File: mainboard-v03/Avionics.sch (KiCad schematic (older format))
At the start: 42 parts, among them J10 Conn_01x03, J8 Conn_01x09, J9 Conn_01x05, SW1 KMR231NG LFS, U1 MAX706RS-T, U2 ATSAMD51J20A-AU, U3 LSM9DS1, Y1 32.768kHz

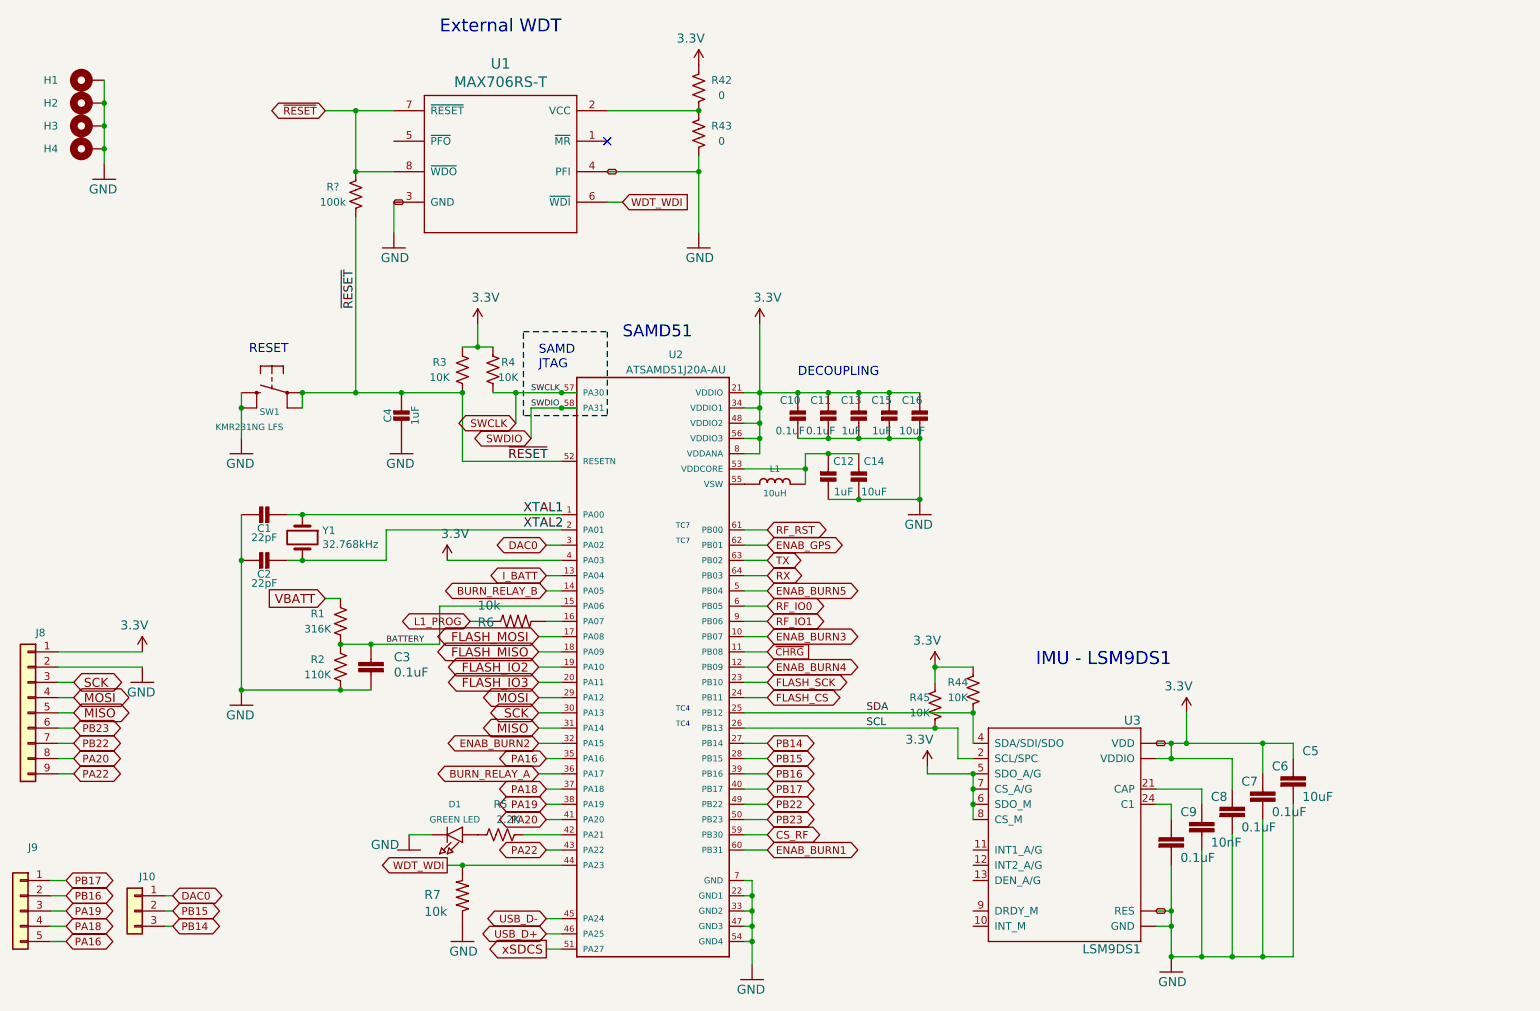
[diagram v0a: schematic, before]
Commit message: schematic organizing
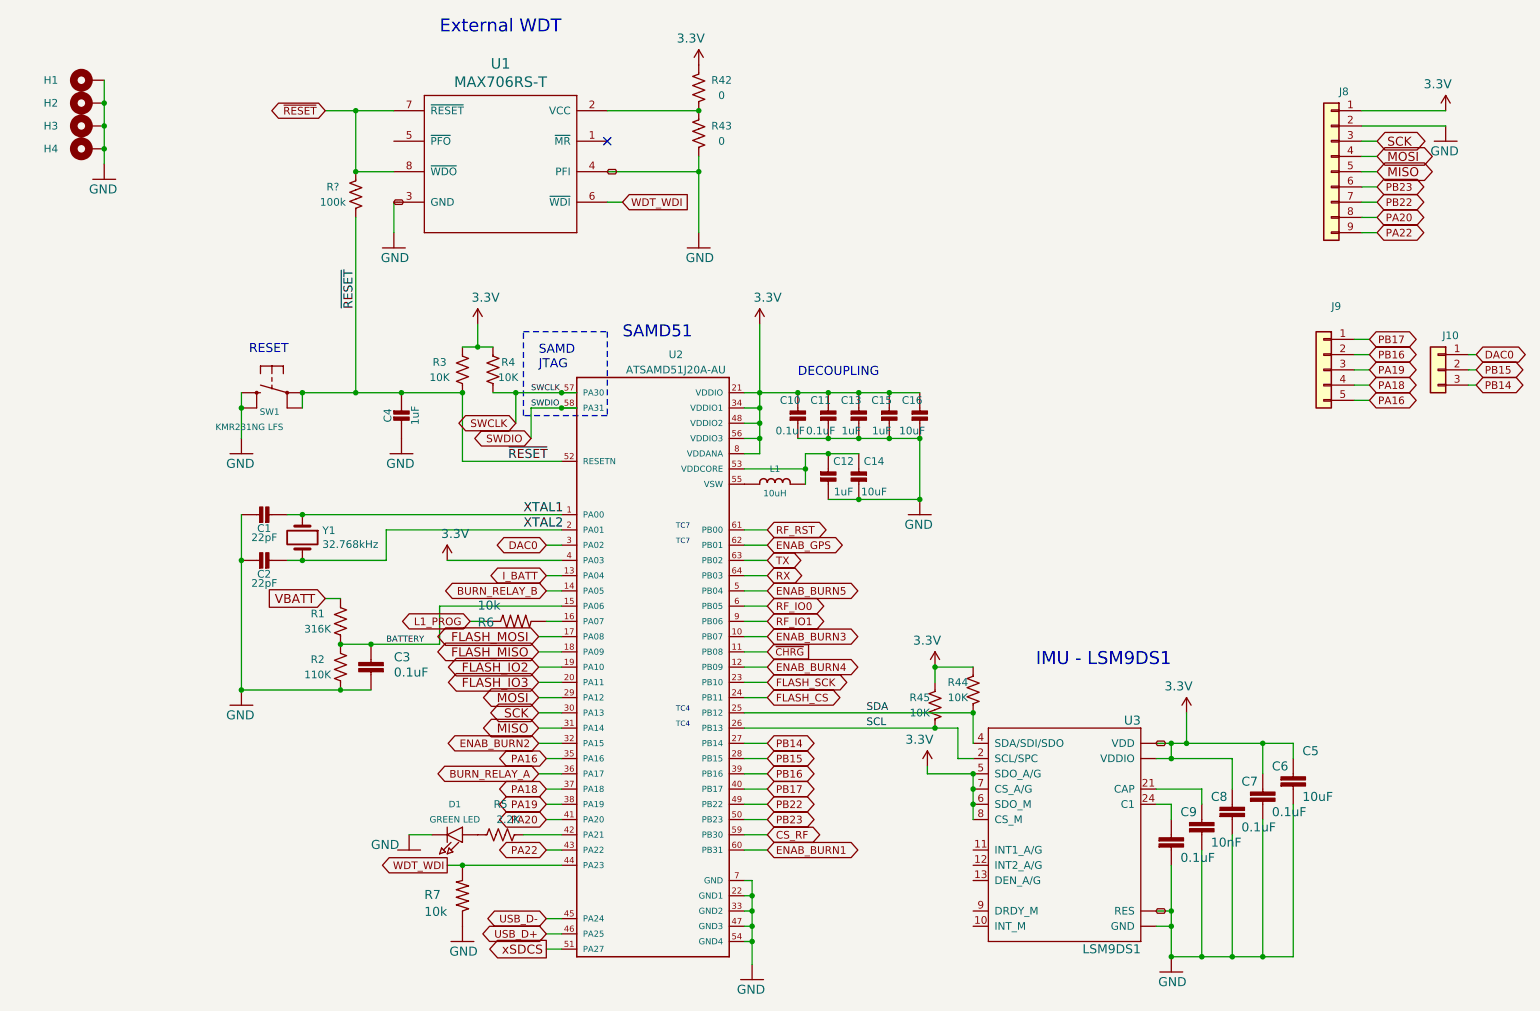
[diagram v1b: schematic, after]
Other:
- moved on the sheet: J10, J8, J9
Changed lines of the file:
@@
 Text GLabel 4600 5850 0    50   BiDi ~ 0
 PA19
-Text GLabel 1500 5150 2    59   BiDi ~ 0
+Text GLabel 10050 1600 2    59   BiDi ~ 0
 MOSI
-Text GLabel 1500 5050 2    59   BiDi ~ 0
+Text GLabel 10050 1500 2    59   BiDi ~ 0
 SCK
-Text GLabel 1500 5250 2    59   BiDi ~ 0
+Text GLabel 10050 1700 2    59   BiDi ~ 0
 MISO
 Wire Wire Line
-	1500 5150 1400 5150
-Wire Wire Line
-	1500 5050 1400 5050
-Wire Wire Line
-	1500 5250 1400 5250
+	10050 1600 9950 1600
+Wire Wire Line
+	10050 1500 9950 1500
+Wire Wire Line
+	10050 1700 9950 1700
 Wire Wire Line
 	6050 4850 5900 4850
@@
 	3350 1300 3150 1300
 Wire Wire Line
-	1400 5550 1500 5550
-Text GLabel 1500 5550 2    50   BiDi ~ 0
+	9950 2000 10050 2000
+Text GLabel 10050 2000 2    50   BiDi ~ 0
 PA20
 Wire Wire Line
-	1400 5650 1500 5650
-Text GLabel 1500 5650 2    50   BiDi ~ 0
+	9950 2100 10050 2100
+Text GLabel 10050 2100 2    50   BiDi ~ 0
 PA22
 Wire Wire Line
-	1400 5350 1500 5350
-Text GLabel 1500 5350 2    50   BiDi ~ 0
+	9950 1800 10050 1800
+Text GLabel 10050 1800 2    50   BiDi ~ 0
 PB23
 Wire Wire Line
-	1400 5450 1500 5450
-Text GLabel 1500 5450 2    50   BiDi ~ 0
+	9950 1900 10050 1900
+Text GLabel 10050 1900 2    50   BiDi ~ 0
 PB22
 $Comp
 L Connector_Generic:Conn_01x09 J8
 U 1 1 5D3643AA
-P 1200 5250
-F 0 "J8" H 1118 5775 50  0000 C CNN
-F 1 "Conn_01x09" H 1118 5776 50  0001 C CNN
-F 2 "Connector_PinHeader_2.54mm:PinHeader_1x09_P2.54mm_Vertical" H 1200 5250 50  0001 C CNN
-F 3 "~" H 1200 5250 50  0001 C CNN
-	1    1200 5250
+P 9750 1700
+F 0 "J8" H 9668 2225 50  0000 C CNN
+F 1 "Conn_01x09" H 9668 2226 50  0001 C CNN
+F 2 "Connector_PinHeader_2.54mm:PinHeader_1x09_P2.54mm_Vertical" H 9750 1700 50  0001 C CNN
+F 3 "~" H 9750 1700 50  0001 C CNN
+	1    9750 1700
 	-1   0    0    -1
 $EndComp
@@
 L mainboard:3.3V #SUPPLY?
 U 1 0 5D370A56
-P 1950 4850
+P 10500 1300
 AR Path="/5D370A56" Ref="#SUPPLY?"  Part="1"
 AR Path="/5CEC5A72/5D370A56" Ref="#SUPPLY0111"  Part="1"
-F 0 "#SUPPLY0111" H 1950 4850 50  0001 C CNN
-F 1 "3.3V" H 1910 4990 59  0000 L BNN
-F 2 "" H 1950 4850 50  0001 C CNN
-F 3 "" H 1950 4850 50  0001 C CNN
-	1    1950 4850
+F 0 "#SUPPLY0111" H 10500 1300 50  0001 C CNN
+F 1 "3.3V" H 10460 1440 59  0000 L BNN
+F 2 "" H 10500 1300 50  0001 C CNN
+F 3 "" H 10500 1300 50  0001 C CNN
+	1    10500 1300
 	-1   0    0    -1
 $EndComp
@@
 L mainboard:GND #GND?
 U 1 0 5D3722F9
-P 1950 5050
+P 10500 1500
 AR Path="/5D3722F9" Ref="#GND?"  Part="1"
 AR Path="/5CEC5A72/5D3722F9" Ref="#GND0101"  Part="1"
-F 0 "#GND0101" H 1950 5050 50  0001 C CNN
-F 1 "GND" H 1850 4950 59  0000 L BNN
-F 2 "" H 1950 5050 50  0001 C CNN
-F 3 "" H 1950 5050 50  0001 C CNN
-	1    1950 5050
+F 0 "#GND0101" H 10500 1500 50  0001 C CNN
+F 1 "GND" H 10400 1400 59  0000 L BNN
+F 2 "" H 10500 1500 50  0001 C CNN
+F 3 "" H 10500 1500 50  0001 C CNN
+	1    10500 1500
 	1    0    0    -1
 $EndComp
 Wire Wire Line
-	1400 4950 1950 4950
-Wire Wire Line
-	1950 4850 1400 4850
+	9950 1400 10500 1400
+Wire Wire Line
+	10500 1300 9950 1300
 Wire Wire Line
 	4700 4150 4600 4150
@@
 L Connector_Generic:Conn_01x05 J9
 U 1 1 5D408200
-P 1150 6550
-F 0 "J9" H 1068 6967 50  0000 C CNN
-F 1 "Conn_01x05" V 1068 6876 50  0001 C CNN
-F 2 "Connector_PinHeader_2.54mm:PinHeader_1x05_P2.54mm_Vertical" H 1150 6550 50  0001 C CNN
-F 3 "~" H 1150 6550 50  0001 C CNN
-	1    1150 6550
-	-1   0    0    -1
-$EndComp
-Wire Wire Line
-	1350 6350 1450 6350
-Text GLabel 1450 6350 2    50   BiDi ~ 0
+P 9700 3000
+F 0 "J9" H 9618 3417 50  0000 C CNN
+F 1 "Conn_01x05" V 9618 3326 50  0001 C CNN
+F 2 "Connector_PinHeader_2.54mm:PinHeader_1x05_P2.54mm_Vertical" H 9700 3000 50  0001 C CNN
+F 3 "~" H 9700 3000 50  0001 C CNN
+	1    9700 3000
+	-1   0    0    -1
+$EndComp
+Wire Wire Line
+	9900 2800 10000 2800
+Text GLabel 10000 2800 2    50   BiDi ~ 0
 PB17
 Wire Wire Line
-	1350 6450 1450 6450
-Text GLabel 1450 6450 2    50   BiDi ~ 0
+	9900 2900 10000 2900
+Text GLabel 10000 2900 2    50   BiDi ~ 0
 PB16
 Wire Wire Line
-	1350 6650 1450 6650
-Wire Wire Line
-	1350 6750 1450 6750
-Text GLabel 1450 6750 2    50   BiDi ~ 0
+	9900 3100 10000 3100
+Wire Wire Line
+	9900 3200 10000 3200
+Text GLabel 10000 3200 2    50   BiDi ~ 0
 PA16
 Wire Wire Line
-	1350 6550 1450 6550
+	9900 3000 10000 3000
 $Comp
 L Mechanical:MountingHole_Pad H1
@@
 L Connector_Generic:Conn_01x03 J10
 U 1 1 5D538CE6
-P 1900 6550
-F 0 "J10" H 1818 6775 50  0000 C CNN
-F 1 "Conn_01x03" H 1818 6776 50  0001 C CNN
-F 2 "Connector_PinHeader_2.54mm:PinHeader_1x03_P2.54mm_Vertical" H 1900 6550 50  0001 C CNN
-F 3 "~" H 1900 6550 50  0001 C CNN
-	1    1900 6550
-	-1   0    0    -1
-$EndComp
-Wire Wire Line
-	2100 6450 2150 6450
-Text GLabel 2150 6450 2    50   BiDi ~ 0
+P 10450 3000
+F 0 "J10" H 10368 3225 50  0000 C CNN
+F 1 "Conn_01x03" H 10368 3226 50  0001 C CNN
+F 2 "Connector_PinHeader_2.54mm:PinHeader_1x03_P2.54mm_Vertical" H 10450 3000 50  0001 C CNN
+F 3 "~" H 10450 3000 50  0001 C CNN
+	1    10450 3000
+	-1   0    0    -1
+$EndComp
+Wire Wire Line
+	10650 2900 10700 2900
+Text GLabel 10700 2900 2    50   BiDi ~ 0
 DAC0
 Wire Wire Line
-	2100 6650 2150 6650
-Text GLabel 2150 6650 2    50   BiDi ~ 0
+	10650 3100 10700 3100
+Text GLabel 10700 3100 2    50   BiDi ~ 0
 PB14
 Wire Wire Line
-	2100 6550 2150 6550
-Text GLabel 2150 6550 2    50   BiDi ~ 0
+	10650 3000 10700 3000
+Text GLabel 10700 3000 2    50   BiDi ~ 0
 PB15
 Wire Wire Line
@@
 Text GLabel 6050 5950 2    50   BiDi ~ 0
 PB23
-Text GLabel 1450 6650 2    50   BiDi ~ 0
+Text GLabel 10000 3100 2    50   BiDi ~ 0
 PA18
-Text GLabel 1450 6550 2    50   BiDi ~ 0
+Text GLabel 10000 3000 2    50   BiDi ~ 0
 PA19
 Wire Wire Line
